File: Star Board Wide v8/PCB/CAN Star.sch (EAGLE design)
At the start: 43 parts

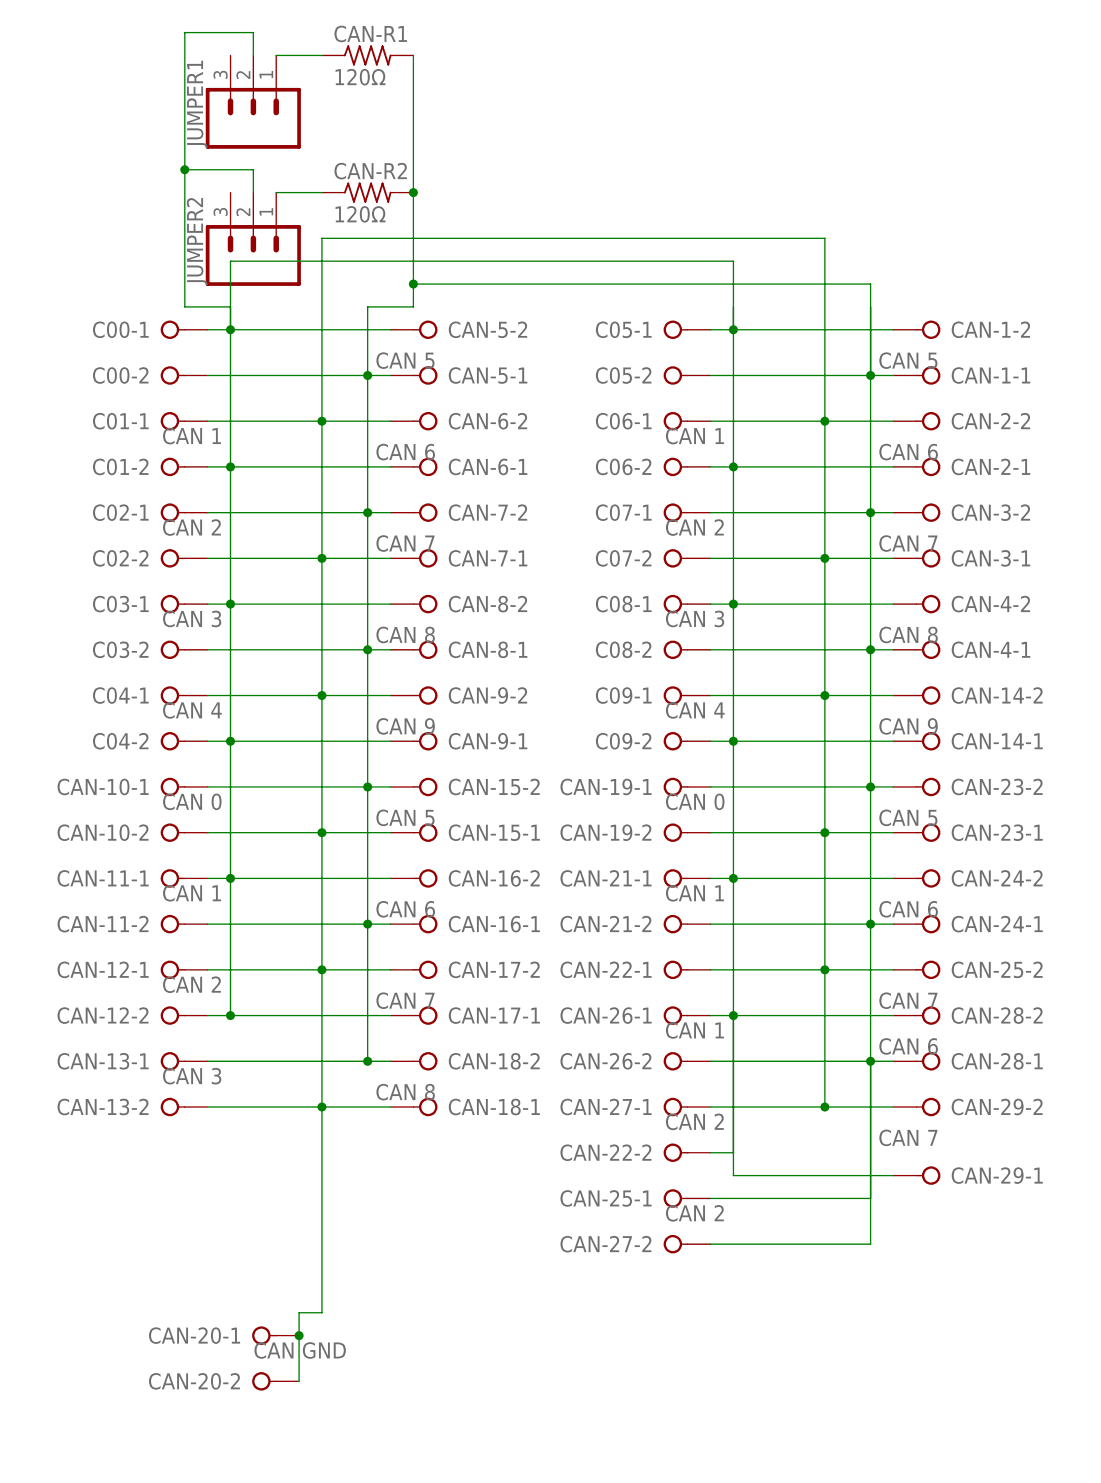
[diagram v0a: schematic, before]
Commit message: Remade board wide v9
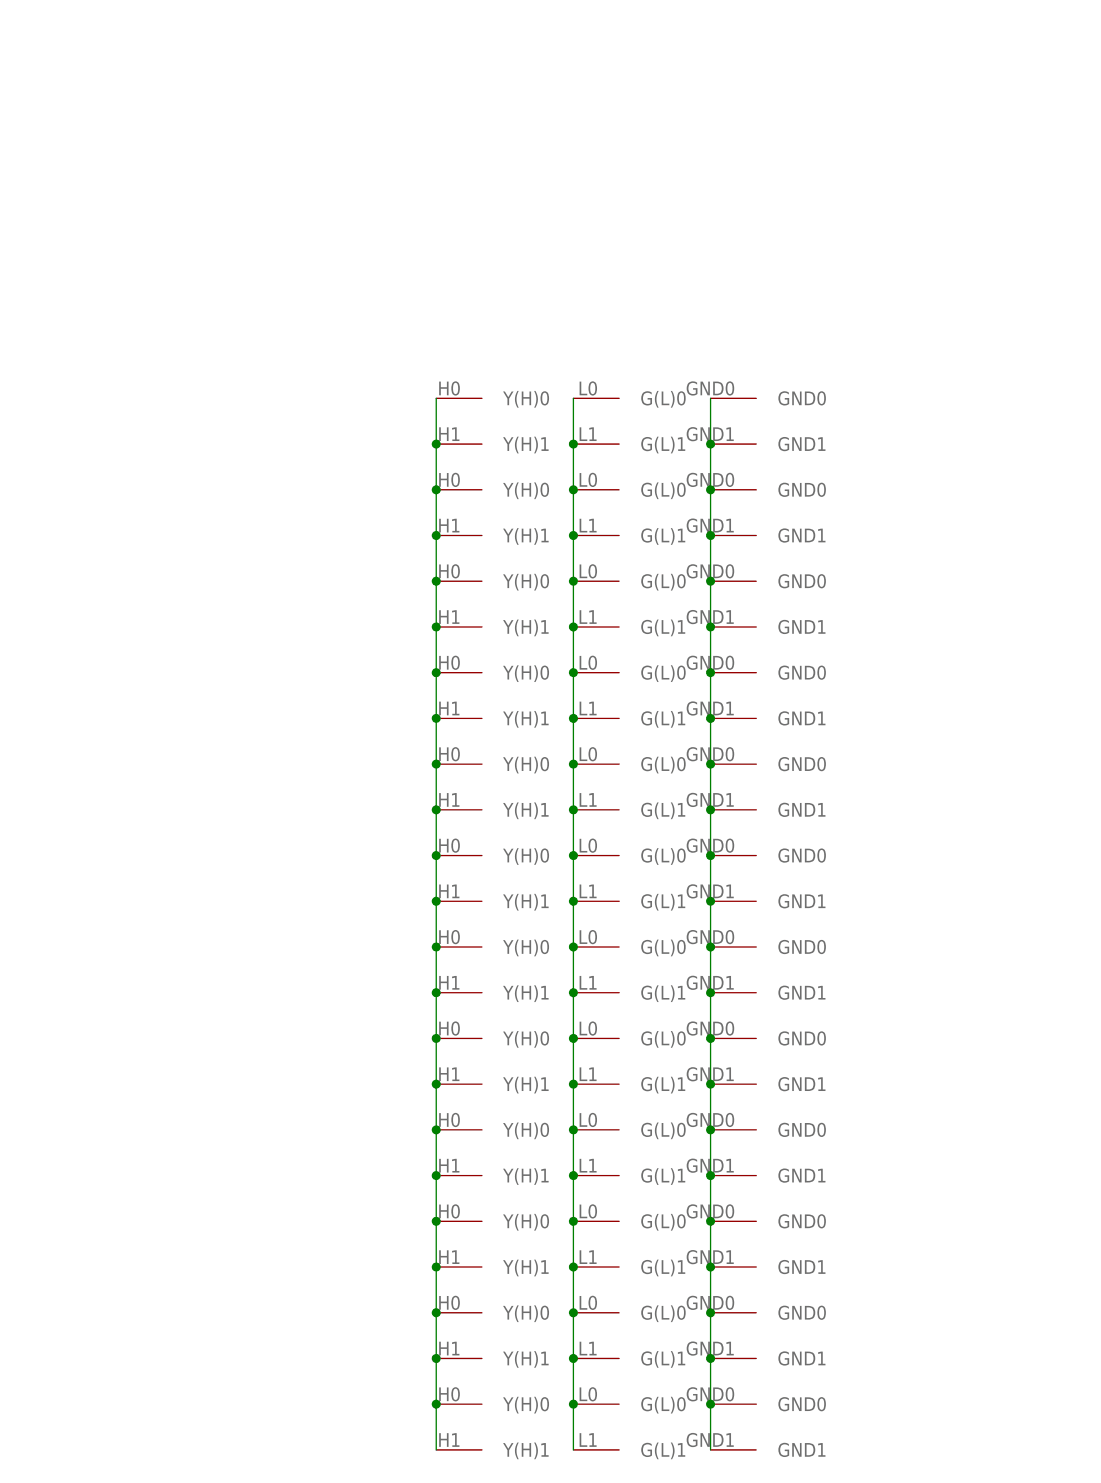
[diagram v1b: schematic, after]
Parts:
- removed C00, C05: (no value), con-wago-508:W237-02P
- removed C01, C06, CAN-11, CAN-21, CAN-26: CAN 1, con-wago-508:W237-02P
- removed C02, C07, CAN-12, CAN-22, CAN-27: CAN 2, con-wago-508:W237-02P
- removed C03, C08, CAN-13: CAN 3, con-wago-508:W237-02P
- removed C04, C09: CAN 4, con-wago-508:W237-02P
- removed CAN-1, CAN-15, CAN-23, CAN-5: CAN 5, con-wago-508:W237-02P
- removed CAN-10, CAN-19: CAN 0, con-wago-508:W237-02P
- removed CAN-14, CAN-9: CAN 9, con-wago-508:W237-02P
- removed CAN-16, CAN-2, CAN-24, CAN-28, CAN-6: CAN 6, con-wago-508:W237-02P
- removed CAN-17, CAN-25, CAN-29, CAN-3, CAN-7: CAN 7, con-wago-508:W237-02P
- removed CAN-18, CAN-4, CAN-8: CAN 8, con-wago-508:W237-02P
- removed CAN-20: CAN GND, con-wago-508:W237-02P
- removed CAN-R1, CAN-R2: 120Ω, resistor:R-US_0207/10
- removed JUMPER1, JUMPER2: (no value), SparkFun-Connectors:CONN_03
- added U$1, U$10, U$11, U$12, U$2, U$3, U$4, U$5, U$6, U$7, U$8, U$9: 2-3-TERMS, custom:2-3-TERMS
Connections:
- removed net G: C00-2.KL, C02-1.KL, C03-2.KL, C05-2.KL, C07-1.KL, C08-2.KL, CAN-1-1.KL, CAN-10-1.KL, CAN-11-2.KL, CAN-13-1.KL, CAN-15-2.KL, CAN-16-1.KL, CAN-18-2.KL, CAN-19-1.KL, CAN-21-2.KL, CAN-23-2.KL, CAN-24-1.KL, CAN-25-1.KL, CAN-26-2.KL, CAN-27-2.KL, CAN-28-1.KL, CAN-3-2.KL, CAN-4-1.KL, CAN-5-1.KL, CAN-7-2.KL, CAN-8-1.KL, CAN-R1.2, CAN-R2.2
- removed net N$1: CAN-R1.1, JUMPER1.1
- removed net N$2: CAN-R2.1, JUMPER2.1
- removed net Y: C00-1.KL, C01-2.KL, C03-1.KL, C04-2.KL, C05-1.KL, C06-2.KL, C08-1.KL, C09-2.KL, CAN-1-2.KL, CAN-11-1.KL, CAN-12-2.KL, CAN-14-1.KL, CAN-16-2.KL, CAN-17-1.KL, CAN-2-1.KL, CAN-21-1.KL, CAN-22-2.KL, CAN-24-2.KL, CAN-26-1.KL, CAN-28-2.KL, CAN-29-1.KL, CAN-4-2.KL, CAN-5-2.KL, CAN-6-1.KL, CAN-8-2.KL, CAN-9-1.KL, JUMPER1.2, JUMPER2.2
- new net G(L): U$1.G(L)0, U$1.G(L)1, U$10.G(L)0, U$10.G(L)1, U$11.G(L)0, U$11.G(L)1, U$12.G(L)0, U$12.G(L)1, U$2.G(L)0, U$2.G(L)1, U$3.G(L)0, U$3.G(L)1, U$4.G(L)0, U$4.G(L)1, U$5.G(L)0, U$5.G(L)1, U$6.G(L)0, U$6.G(L)1, U$7.G(L)0, U$7.G(L)1, U$8.G(L)0, U$8.G(L)1, U$9.G(L)0, U$9.G(L)1
- new net Y(H): U$1.Y(H)0, U$1.Y(H)1, U$10.Y(H)0, U$10.Y(H)1, U$11.Y(H)0, U$11.Y(H)1, U$12.Y(H)0, U$12.Y(H)1, U$2.Y(H)0, U$2.Y(H)1, U$3.Y(H)0, U$3.Y(H)1, U$4.Y(H)0, U$4.Y(H)1, U$5.Y(H)0, U$5.Y(H)1, U$6.Y(H)0, U$6.Y(H)1, U$7.Y(H)0, U$7.Y(H)1, U$8.Y(H)0, U$8.Y(H)1, U$9.Y(H)0, U$9.Y(H)1
- net GND: now also U$1.GND0, U$1.GND1, U$10.GND0, U$10.GND1, U$11.GND0, U$11.GND1, U$12.GND0, U$12.GND1, U$2.GND0, U$2.GND1, U$3.GND0, U$3.GND1, U$4.GND0, U$4.GND1, U$5.GND0, U$5.GND1, U$6.GND0, U$6.GND1, U$7.GND0, U$7.GND1, U$8.GND0, U$8.GND1, U$9.GND0, U$9.GND1; no longer C01-1.KL, C02-2.KL, C04-1.KL, C06-1.KL, C07-2.KL, C09-1.KL, CAN-10-2.KL, CAN-12-1.KL, CAN-13-2.KL, CAN-14-2.KL, CAN-15-1.KL, CAN-17-2.KL, CAN-18-1.KL, CAN-19-2.KL, CAN-2-2.KL, CAN-20-1.KL, CAN-20-2.KL, CAN-22-1.KL, CAN-23-1.KL, CAN-25-2.KL, CAN-27-1.KL, CAN-29-2.KL, CAN-3-1.KL, CAN-6-2.KL, CAN-7-1.KL, CAN-9-2.KL
